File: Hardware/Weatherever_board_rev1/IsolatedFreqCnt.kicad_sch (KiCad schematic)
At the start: 25 parts, among them J1 ProbeConn, U1 ZXCT1009F, U301 6N137, U302 LM393, U303 6N137

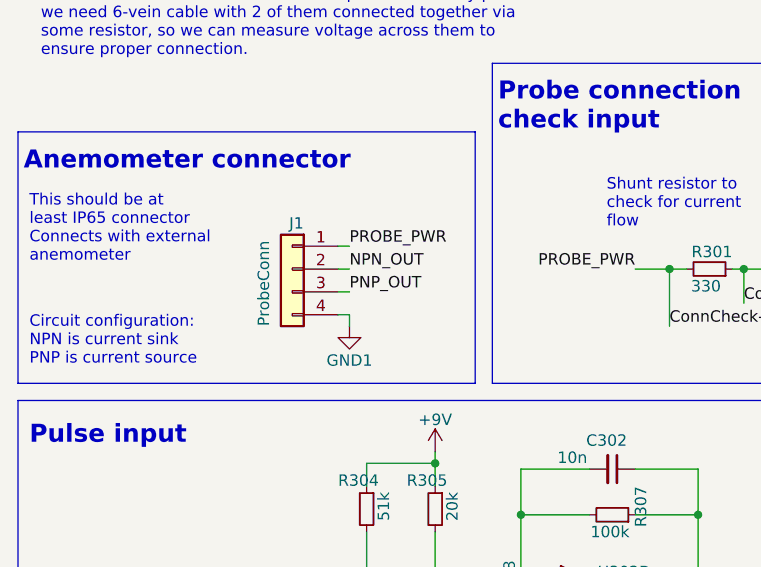
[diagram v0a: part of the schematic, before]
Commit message: Layout impl start
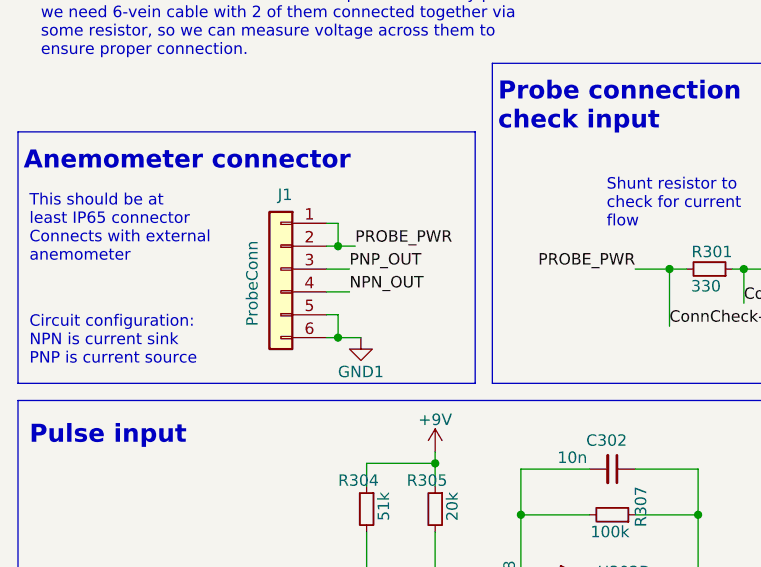
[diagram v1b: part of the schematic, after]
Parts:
- J1: footprint (none) -> Connector_IDC:IDC-Header_2x03_P2.54mm_Vertical; symbol Connector_Generic:Conn_01x04 -> Connector_Generic:Conn_01x06
- R301: footprint (none) -> Resistor_SMD:R_0805_2012Metric_Pad1.20x1.40mm_HandSolder
- U301, U303: footprint Package_DIP:SMDIP-6_W7.62mm -> Package_DIP:SMDIP-8_W7.62mm
- U302: footprint (none) -> Package_SO:SO-8_3.9x4.9mm_P1.27mm
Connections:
- net ConnCheck-: now also J1.2 (Pin_2)
- net GND1: now also J1.5 (Pin_5), J1.6 (Pin_6); no longer J1.4 (Pin_4)
- net NPN_OUT: now also J1.4 (Pin_4); no longer J1.2 (Pin_2)
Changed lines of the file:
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@@
   (junction (at 74.93 74.295) (diameter 0) (color 0 0 0 0)
   )
+  (junction (at 64.135 50.165) (diameter 0) (color 0 0 0 0)
+  )
   (junction (at 100.965 52.705) (diameter 0) (color 0 0 0 0)
   )
   (junction (at 104.14 90.805) (diameter 0) (color 0 0 0 0)
   )
+  (junction (at 64.135 60.325) (diameter 0) (color 0 0 0 0)
+  )
   (junction (at 109.22 52.705) (diameter 0) (color 0 0 0 0)
   )
@@
     (stroke (width 0) (type default))
   )
-  (wire (pts (xy 65.405 55.245) (xy 64.135 55.245))
+  (wire (pts (xy 65.405 55.245) (xy 62.865 55.245))
     (stroke (width 0) (type default))
   )
@@
     (stroke (width 0) (type default))
   )
-  (wire (pts (xy 65.405 52.705) (xy 64.135 52.705))
+  (wire (pts (xy 65.405 52.705) (xy 62.865 52.705))
     (stroke (width 0) (type default))
   )
@@
     (stroke (width 0) (type default))
   )
-  (wire (pts (xy 64.135 57.785) (xy 65.405 57.785))
+  (wire (pts (xy 62.865 57.785) (xy 64.135 57.785))
     (stroke (width 0) (type default))
   )
@@
     (stroke (width 0) (type default))
   )
+  (wire (pts (xy 62.865 60.325) (xy 64.135 60.325))
+    (stroke (width 0) (type default))
+  )
   (wire (pts (xy 107.95 52.705) (xy 109.22 52.705))
     (stroke (width 0) (type default))
@@
     (stroke (width 0) (type default))
   )
+  (wire (pts (xy 64.135 47.625) (xy 64.135 50.165))
+    (stroke (width 0) (type default))
+  )
   (wire (pts (xy 148.59 67.31) (xy 152.4 67.31))
     (stroke (width 0) (type default))
@@
     (stroke (width 0) (type default))
   )
+  (wire (pts (xy 64.135 60.325) (xy 66.675 60.325))
+    (stroke (width 0) (type default))
+  )
+  (wire (pts (xy 64.135 47.625) (xy 62.865 47.625))
+    (stroke (width 0) (type default))
+  )
   (wire (pts (xy 146.685 120.65) (xy 146.685 123.19))
     (stroke (width 0) (type default))
@@
     (stroke (width 0) (type default))
   )
+  (wire (pts (xy 64.135 57.785) (xy 64.135 60.325))
+    (stroke (width 0) (type default))
+  )
   (polyline (pts (xy 127 111.76) (xy 28.575 111.76))
     (stroke (width 0) (type default))
@@
     (stroke (width 0) (type default))
   )
-  (wire (pts (xy 64.135 50.165) (xy 65.405 50.165))
+  (wire (pts (xy 62.865 50.165) (xy 64.135 50.165))
     (stroke (width 0) (type default))
   )
@@
     (stroke (width 0) (type default))
   )
-  (wire (pts (xy 65.405 57.785) (xy 65.405 59.055))
-    (stroke (width 0) (type default))
-  )
   (wire (pts (xy 93.345 123.825) (xy 84.455 123.825))
     (stroke (width 0) (type default))
@@
   )
   (wire (pts (xy 118.745 123.19) (xy 120.015 123.19))
+    (stroke (width 0) (type default))
+  )
+  (wire (pts (xy 64.135 50.165) (xy 66.04 50.165))
     (stroke (width 0) (type default))
   )
@@
     (effects (font (size 1.27 1.27)) (justify right bottom))
   )
-  (label "PNP_OUT" (at 65.405 55.245 0) (fields_autoplaced)
+  (label "PNP_OUT" (at 65.405 52.705 0) (fields_autoplaced)
     (effects (font (size 1.27 1.27)) (justify left bottom))
   )
@@
     (effects (font (size 1.27 1.27)) (justify left bottom))
   )
-  (label "PROBE_PWR" (at 65.405 50.165 0) (fields_autoplaced)
+  (label "PROBE_PWR" (at 66.04 50.165 0) (fields_autoplaced)
     (effects (font (size 1.27 1.27)) (justify left bottom))
   )
@@
     (effects (font (size 1.27 1.27)) (justify right bottom))
   )
-  (label "NPN_OUT" (at 65.405 52.705 0) (fields_autoplaced)
+  (label "NPN_OUT" (at 65.405 55.245 0) (fields_autoplaced)
     (effects (font (size 1.27 1.27)) (justify left bottom))
   )
@@
       (effects (font (size 1.27 1.27)))
     )
-    (property "Footprint" "Package_DIP:SMDIP-6_W7.62mm" (at 133.985 95.885 0)
+    (property "Footprint" "Package_DIP:SMDIP-8_W7.62mm" (at 133.985 95.885 0)
       (effects (font (size 1.27 1.27)) hide)
     )
@@
       (effects (font (size 1.27 1.27)))
     )
-    (property "Footprint" "Package_DIP:SMDIP-6_W7.62mm" (at 133.985 135.89 0)
+    (property "Footprint" "Package_DIP:SMDIP-8_W7.62mm" (at 133.985 135.89 0)
       (effects (font (size 1.27 1.27)) hide)
     )
@@
       (effects (font (size 1.27 1.27)))
     )
-    (property "Footprint" "" (at 93.98 134.62 0)
+    (property "Footprint" "Package_SO:SO-8_3.9x4.9mm_P1.27mm" (at 93.98 134.62 0)
       (effects (font (size 1.27 1.27)) hide)
     )
@@
       (effects (font (size 1.27 1.27)) (justify right))
     )
-    (property "Footprint" "" (at 105.41 52.705 0)
+    (property "Footprint" "Resistor_SMD:R_0805_2012Metric_Pad1.20x1.40mm_HandSolder" (at 105.41 52.705 0)
       (effects (font (size 1.27 1.27)) hide)
     )
@@
       (effects (font (size 1.27 1.27)))
     )
-    (property "Footprint" "" (at 93.98 90.805 0)
+    (property "Footprint" "Package_SO:SO-8_3.9x4.9mm_P1.27mm" (at 93.98 90.805 0)
       (effects (font (size 1.27 1.27)) hide)
     )
@@
     )
   )
-  (symbol (lib_id "power:GND1") (at 65.405 59.055 0) (unit 1)
-    (in_bom yes) (on_board yes) (dnp no)
-    (property "Reference" "#PWR0303" (at 65.405 65.405 0)
-      (effects (font (size 1.27 1.27)) hide)
-    )
-    (property "Value" "GND1" (at 65.405 62.865 0)
-      (effects (font (size 1.27 1.27)))
-    )
-    (property "Footprint" "" (at 65.405 59.055 0)
-      (effects (font (size 1.27 1.27)) hide)
-    )
-    (property "Datasheet" "" (at 65.405 59.055 0)
+  (symbol (lib_id "power:GND1") (at 66.675 60.325 0) (unit 1)
+    (in_bom yes) (on_board yes) (dnp no)
+    (property "Reference" "#PWR0303" (at 66.675 66.675 0)
+      (effects (font (size 1.27 1.27)) hide)
+    )
+    (property "Value" "GND1" (at 66.675 64.135 0)
+      (effects (font (size 1.27 1.27)))
+    )
+    (property "Footprint" "" (at 66.675 60.325 0)
+      (effects (font (size 1.27 1.27)) hide)
+    )
+    (property "Datasheet" "" (at 66.675 60.325 0)
       (effects (font (size 1.27 1.27)) hide)
     )
@@
     )
   )
-  (symbol (lib_id "Connector_Generic:Conn_01x04") (at 59.055 52.705 0) (mirror y) (unit 1)
-    (in_bom yes) (on_board yes) (dnp no)
-    (property "Reference" "J1" (at 60.325 47.625 0)
+  (symbol (lib_id "Connector_Generic:Conn_01x06") (at 57.785 52.705 0) (mirror y) (unit 1)
+    (in_bom yes) (on_board yes) (dnp no)
+    (property "Reference" "J1" (at 59.055 44.45 0)
       (effects (font (size 1.27 1.27)) (justify left))
     )
-    (property "Value" "ProbeConn" (at 55.88 59.055 90)
+    (property "Value" "ProbeConn" (at 54.61 59.055 90)
       (effects (font (size 1.27 1.27)) (justify left))
     )
-    (property "Footprint" "" (at 59.055 52.705 0)
-      (effects (font (size 1.27 1.27)) hide)
-    )
-    (property "Datasheet" "~" (at 59.055 52.705 0)
+    (property "Footprint" "Connector_IDC:IDC-Header_2x03_P2.54mm_Vertical" (at 57.785 52.705 0)
+      (effects (font (size 1.27 1.27)) hide)
+    )
+    (property "Datasheet" "~" (at 57.785 52.705 0)
       (effects (font (size 1.27 1.27)) hide)
     )
@@
     (pin "3")
     (pin "4")
+    (pin "5")
+    (pin "6")
     (instances
       (project "Weatherever_board_rev1"
@@
       (effects (font (size 1.27 1.27)) (justify left))
     )
-    (property "Footprint" "" (at 62.865 179.705 0)
-      (effects (font (size 1.27 1.27)) hide)
-    )
+    (property "Footprint" "Package_SO:SO-8_3.9x4.9mm_P1.27mm" (at 62.865 179.705 0)
+      (effects (font (size 1.27 1.27)) hide)
+    )
